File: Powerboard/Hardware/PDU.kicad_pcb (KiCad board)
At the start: 4 copper layers, 58 x 50 mm, 148 parts, among them IC1 TPS259830ONRGER, IC2 SiC437AED-T1-GE3, J1 Conn_01x03_MountingPin, J2 FAN, J3 USB_C_Receptacle_USB2.0, J4 Conn_01x02_Male, J5 Conn_01x08_Male, J6 Conn_01x02_Male, J7 XT60PW-M, J8 Conn_01x04_Male, J9 XT60PW-M, Q1 SSM3K15AMFV,L3F, Q10 SQS141ELNW-T1_GE3, Q5 PXP012-30QLJ, Q6 PXP012-30QLJ, Q7 SQS141ELNW-T1_GE3, Q8 SQS141ELNW-T1_GE3, Q9 SQS141ELNW-T1_GE3, U1 LTC4412xS6, U10 SC4215, U2 ESP32-S3, U4 MAX77827AEFD+T, U5 SN65HVD230, U6 LTC4412xS6, U7 LTC4412xS6, U8 LTC4412xS6, Y1 40MHz±10ppm

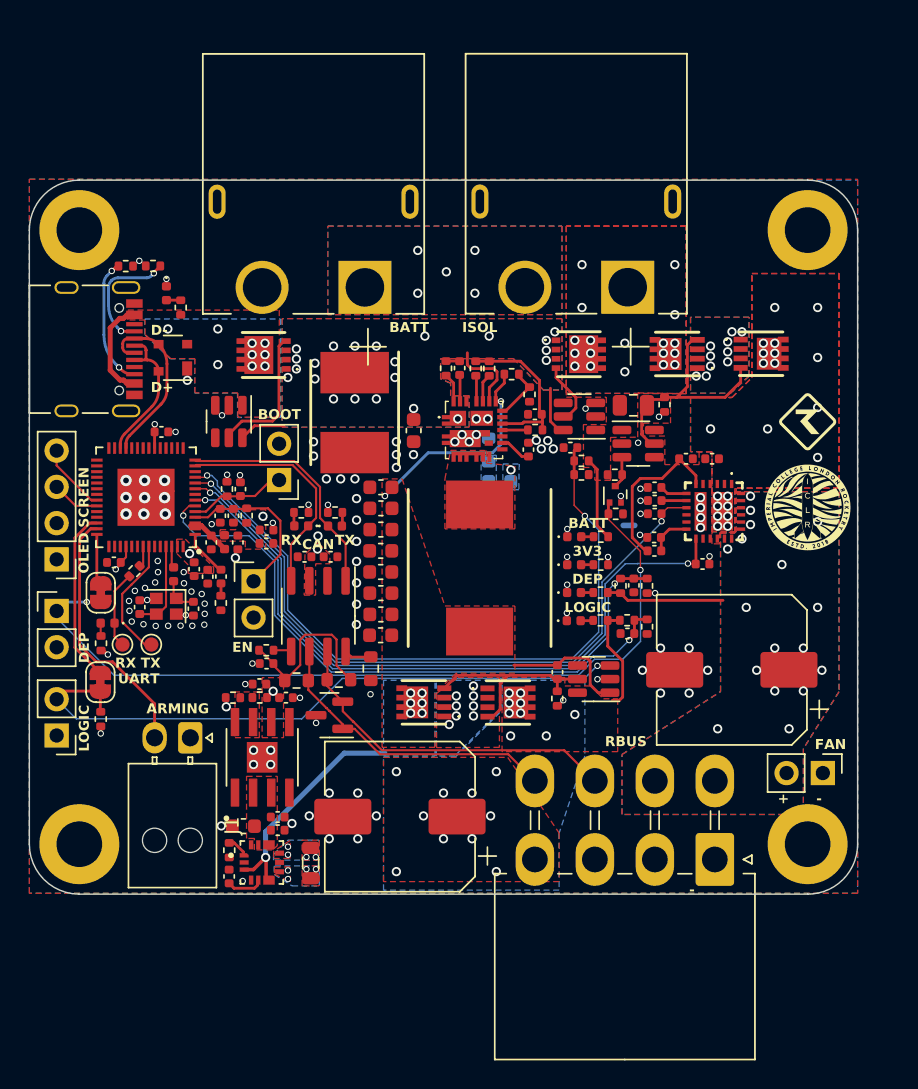
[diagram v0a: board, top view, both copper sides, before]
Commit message: post Andrei review
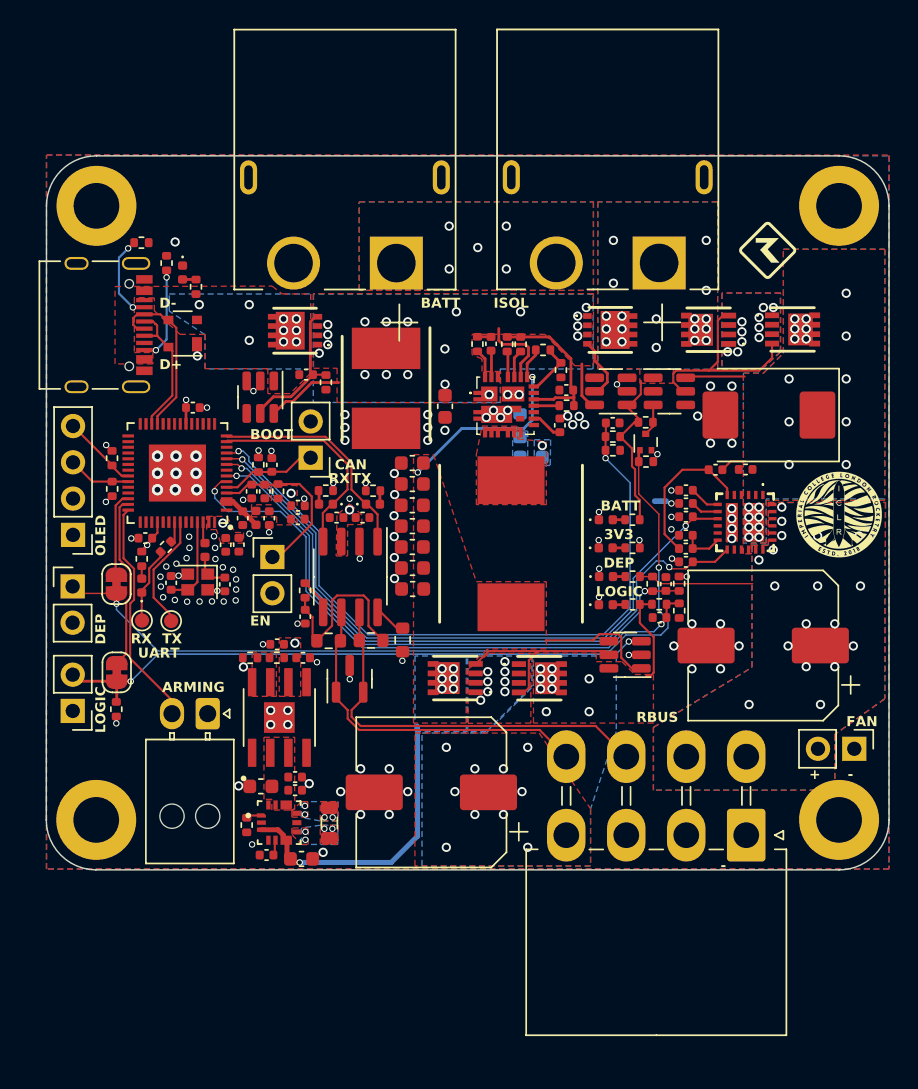
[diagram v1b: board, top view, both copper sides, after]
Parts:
- removed C29: 2.2uF, Capacitor_SMD:C_0402_1005Metric
- removed C31: 2.2uF, Capacitor_SMD:C_0805_2012Metric
- removed R44, R45: 100k, Resistor_SMD:R_0402_1005Metric
- added D4: SMCJ24AHE3_A/H, Diode_SMD:D_SMC, F.Cu at (164.1, 88.6)
- added R46: 2.2k, Resistor_SMD:R_0402_1005Metric, F.Cu at (118.1, 91.6)
- added R47: 100k, Resistor_SMD:R_0402_1005Metric, F.Cu at (133.1, 86.3)
- C12: value DNP -> 2.2uF
- C16: value 680pF -> TBD
- R37: value 5.1 -> TBD
- R42: value 681 -> 680
- R8: value DNP -> 2.2k
- moved C17 22.3 mm to (131.4, 119.7), turned to 0 degrees
- moved C12 15.3 mm to (131.7, 85.8), turned to 0 degrees
- moved G*** 12.3 mm to (164.0, 77.1)
- moved R8 11.0 mm to (118.1, 93.8)
- moved R5 6.56 mm to (120.2, 98.7), turned to -90 degrees
- moved R23 5.00 mm to (131.6, 100.9), turned to -90 degrees
- moved U7 4.27 mm to (157.1, 86.9)
- moved R35 4.26 mm to (155.5, 89.1)
- moved C20 4.25 mm to (131.6, 102.7), turned to -90 degrees
- moved Q1 4.23 mm to (155.5, 90.5)
- moved R34 4.23 mm to (155.5, 91.8)
- moved C34 3.94 mm to (139.1, 100.8)
- moved C30 3.93 mm to (139.1, 99.3)
- moved C52 3.91 mm to (130.9, 113.9)
- moved C32 3.91 mm to (139.1, 97.8)
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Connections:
- C12 pad 1: Net-(C12-Pad1) -> VBUS
- C12 pad 2: Net-(U2-LNA_IN/RF) -> Net-(Q6-G)
- R8 pad 1: GND -> +3V3
- R8 pad 2: Net-(C12-Pad1) -> /SCL
- U2 pad 1: Net-(U2-LNA_IN/RF) -> unconnected-(U2-LNA_IN/RF-Pad1)
- U2 pad 40: /LogicSwitch -> /DepSwitch
- U2 pad 41: /ARMING -> /LogicSwitch
- U2 pad 42: /DepSwitch -> /ARMING
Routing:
- net VBUS: track 7.11 -> 0.00 mm
- net /Switches+RBUS/EFuse_IN: track 0.00 -> 6.00 mm, vias 21 -> 22
- net +12V: track 5.87 -> 11.8 mm
- net RBUS_uC_V: track 40.0 -> 45.0 mm
- net /CAN+: track 24.3 -> 28.2 mm
- net Net-(U2-LNA_IN/RF): track 3.28 -> 0.00 mm
- net Net-(J4-Pin_2): track 45.6 -> 42.6 mm, vias 1 -> 2
- net /CAN-: track 21.4 -> 24.3 mm
- net /EFuse_PG: track 49.4 -> 46.7 mm
- net /DepSwitch: track 3.54 -> 5.96 mm
- net Net-(J3-CC1): track 8.61 -> 6.20 mm
- net Net-(J3-CC2): track 9.07 -> 6.71 mm
- net /ARMING: track 18.2 -> 16.0 mm
- net Net-(IC2-EN): track 12.2 -> 14.2 mm, vias 22 -> 19
- net /DepCurrent: track 48.8 -> 46.7 mm
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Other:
- board size 58 x 50 mm -> 59 x 50 mm
- board text added: "OLED"
- board text added: "RAE 2024 Designed by Artem Sheykin"
- board text added: "x"
- board text removed: "Designed by Artem Sheykin RAE 2024"
- board text removed: "OLED SCREEN"
